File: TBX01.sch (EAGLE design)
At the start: 75 parts, among them IC1 TPS62120, U3 STM32L151CCT6, U6 MCP73833, X2 FH12-10S-0.5SH, Y1 CRYSTAL.ABS07

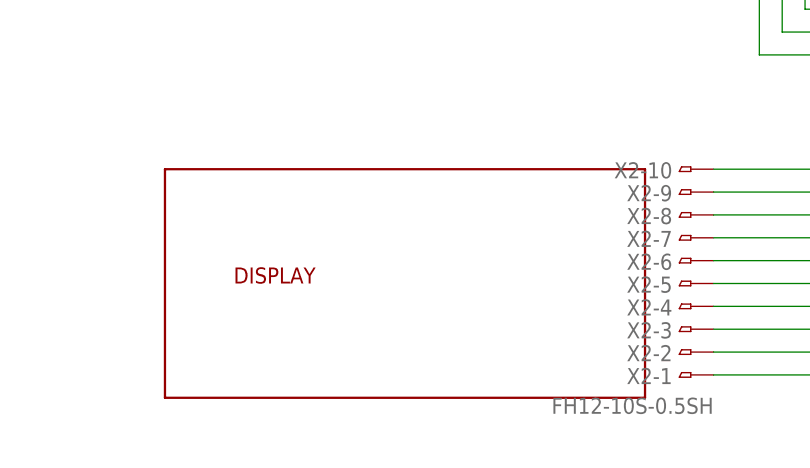
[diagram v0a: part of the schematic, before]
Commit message: TBX01 v0.4
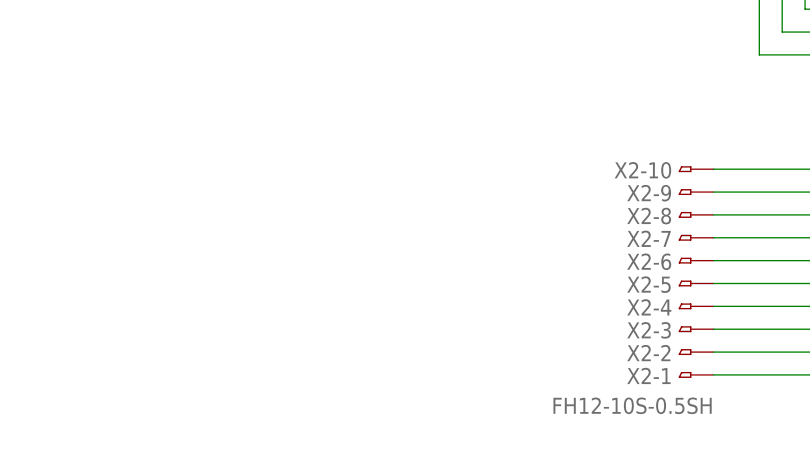
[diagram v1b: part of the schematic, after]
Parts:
- removed U$1: LS013B4DN04, sharp_LCD:LS013B4DN04
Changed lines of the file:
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@@
 <part name="JP1" library="SparkFun-Connectors" deviceset="USB" device="-MICROB"/>
 <part name="X2" library="con-hirose" deviceset="FH12-10S-0.5S" device="H"/>
-<part name="U$1" library="sharp_LCD" deviceset="LS013B4DN04" device=""/>
 <part name="U6" library="microbuilder" deviceset="MCP73833" device="" value="MCP73833"/>
 <part name="FRAME1" library="frames" deviceset="A3L-LOC" device=""/>
@@
 <instance part="X2" gate="-9" x="-124.46" y="-40.64" rot="R180"/>
 <instance part="X2" gate="-10" x="-124.46" y="-38.1" rot="R180"/>
-<instance part="U$1" gate="G$1" x="-182.88" y="-63.5"/>
 <instance part="U6" gate="G$1" x="-86.36" y="154.94"/>
 <instance part="FRAME1" gate="G$1" x="-200.66" y="-73.66"/>
